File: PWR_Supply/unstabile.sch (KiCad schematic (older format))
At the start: 4 parts

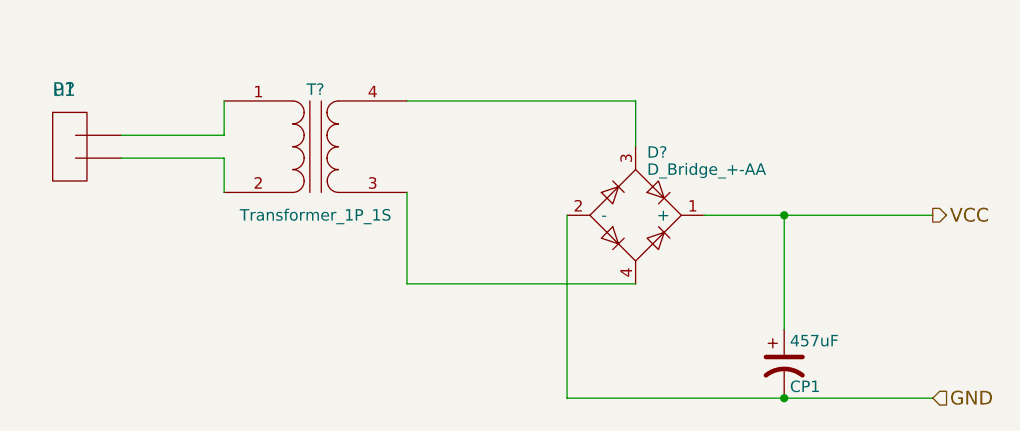
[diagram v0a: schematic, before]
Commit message: single_amp
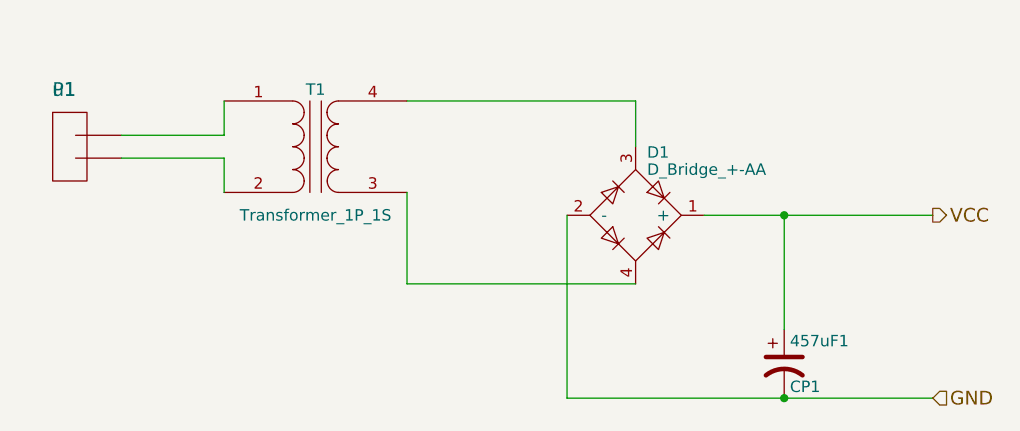
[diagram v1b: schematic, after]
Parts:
- gave numbers to parts that had none: 3
- renumbered 457uF to 457uF1
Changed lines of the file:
@@
 LIBS:contrib
 LIBS:valves
+LIBS:PWR_Supply-cache
 EELAYER 25 0
 EELAYER END
@@
 $EndDescr
 $Comp
-L Transformer_1P_1S T?
+L Transformer_1P_1S T1
 U 1 1 58D279AE
 P 3200 2150
-F 0 "T?" H 3200 2400 50  0000 C CNN
+F 0 "T1" H 3200 2400 50  0000 C CNN
 F 1 "Transformer_1P_1S" H 3200 1850 50  0000 C CNN
 F 2 "" H 3200 2150 50  0000 C CNN
@@
 $EndComp
 $Comp
-L D_Bridge_+-AA D?
+L D_Bridge_+-AA D1
 U 1 1 58D27A8D
 P 4600 2450
-F 0 "D?" H 4650 2725 50  0000 L CNN
+F 0 "D1" H 4650 2725 50  0000 L CNN
 F 1 "D_Bridge_+-AA" H 4650 2650 50  0000 L CNN
 F 2 "" H 4600 2450 50  0000 C CNN
@@
 $EndComp
 $Comp
-L CP1 457uF
+L CP1 457uF1
 U 1 1 58D27AC8
 P 5250 3100
-F 0 "457uF" H 5275 3200 50  0000 L CNN
+F 0 "457uF1" H 5275 3200 50  0000 L CNN
 F 1 "CP1" H 5275 3000 50  0000 L CNN
 F 2 "" H 5250 3100 50  0000 C CNN
@@
 	2800 2200 2800 2350
 $Comp
-L P1 u?
+L P1 u1
 U 1 1 58D2839B
 P 1400 2700
-F 0 "u?" H 2100 3500 60  0000 C CNN
+F 0 "u1" H 2100 3500 60  0000 C CNN
 F 1 "P1" H 2100 3500 60  0000 C CNN
 F 2 "" H 2100 3500 60  0001 C CNN

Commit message: Kursa_darbs_PCB
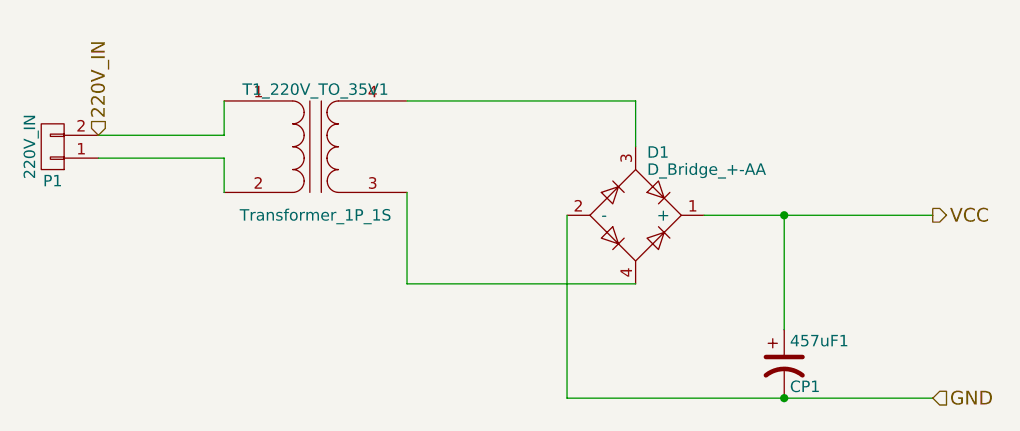
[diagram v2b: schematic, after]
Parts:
- removed u1: P1, symbol P1
- added P1: 220V_IN, symbol CONN_01X02
- renumbered T1 to T1_220V_TO_35V1
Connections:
- net 220V_IN: now reaches T1_220V_TO_35V1.1 (AA)
- net 220V_IN: now also P1.2 (P2)
- net at T1_220V_TO_35V1.2 (AB): now also P1.1 (P1)
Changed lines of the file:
@@
 $EndDescr
 $Comp
-L Transformer_1P_1S T1
+L Transformer_1P_1S T1_220V_TO_35V1
 U 1 1 58D279AE
 P 3200 2150
-F 0 "T1" H 3200 2400 50  0000 C CNN
+F 0 "T1_220V_TO_35V1" H 3200 2400 50  0000 C CNN
 F 1 "Transformer_1P_1S" H 3200 1850 50  0000 C CNN
 F 2 "" H 3200 2150 50  0000 C CNN
@@
 Connection ~ 5250 3250
 Wire Wire Line
-	2800 1950 2800 2100
+	2800 2100 2800 1950
 Wire Wire Line
 	2800 2200 2800 2350
-$Comp
-L P1 u1
-U 1 1 58D2839B
-P 1400 2700
-F 0 "u1" H 2100 3500 60  0000 C CNN
-F 1 "P1" H 2100 3500 60  0000 C CNN
-F 2 "" H 2100 3500 60  0001 C CNN
-F 3 "" H 2100 3500 60  0001 C CNN
-	1    1400 2700
-	1    0    0    -1
-$EndComp
 Wire Wire Line
-	2800 2100 2350 2100
+	2250 2100 2800 2100
 Wire Wire Line
-	2800 2200 2350 2200
+	2250 2200 2800 2200
 Text HLabel 5900 2450 2    60   Output ~ 0
 VCC
 Text HLabel 5900 3250 2    60   Input ~ 0
 GND
+$Comp
+L CONN_01X02 P1
+U 1 1 5943C2B3
+P 2050 2150
+F 0 "P1" H 2050 2300 50  0000 C CNN
+F 1 "220V_IN" V 2150 2150 50  0000 C CNN
+F 2 "" H 2050 2150 50  0000 C CNN
+F 3 "" H 2050 2150 50  0000 C CNN
+	1    2050 2150
+	-1   0    0    1
+$EndComp
+Text HLabel 2250 2100 1    60   Input ~ 0
+220V_IN
 $EndSCHEMATC
